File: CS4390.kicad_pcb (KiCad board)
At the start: 2 copper layers, 97.3 x 51.6 mm, 53 parts, among them J1 Power In, J2 Audio Out, J3 Data In, U1 CS4390, U2 OPA2604, U3 DRV134, U4 DRV134

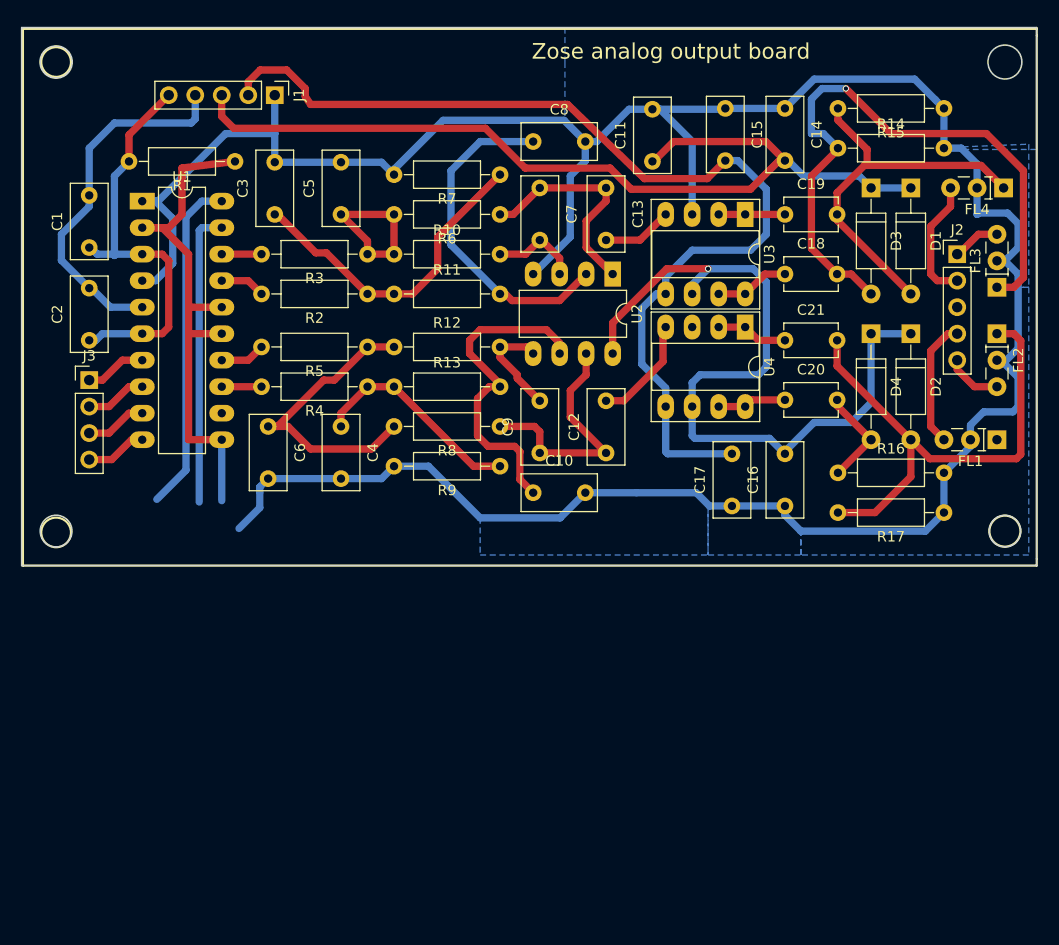
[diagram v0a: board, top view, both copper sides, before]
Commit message: pre-trace
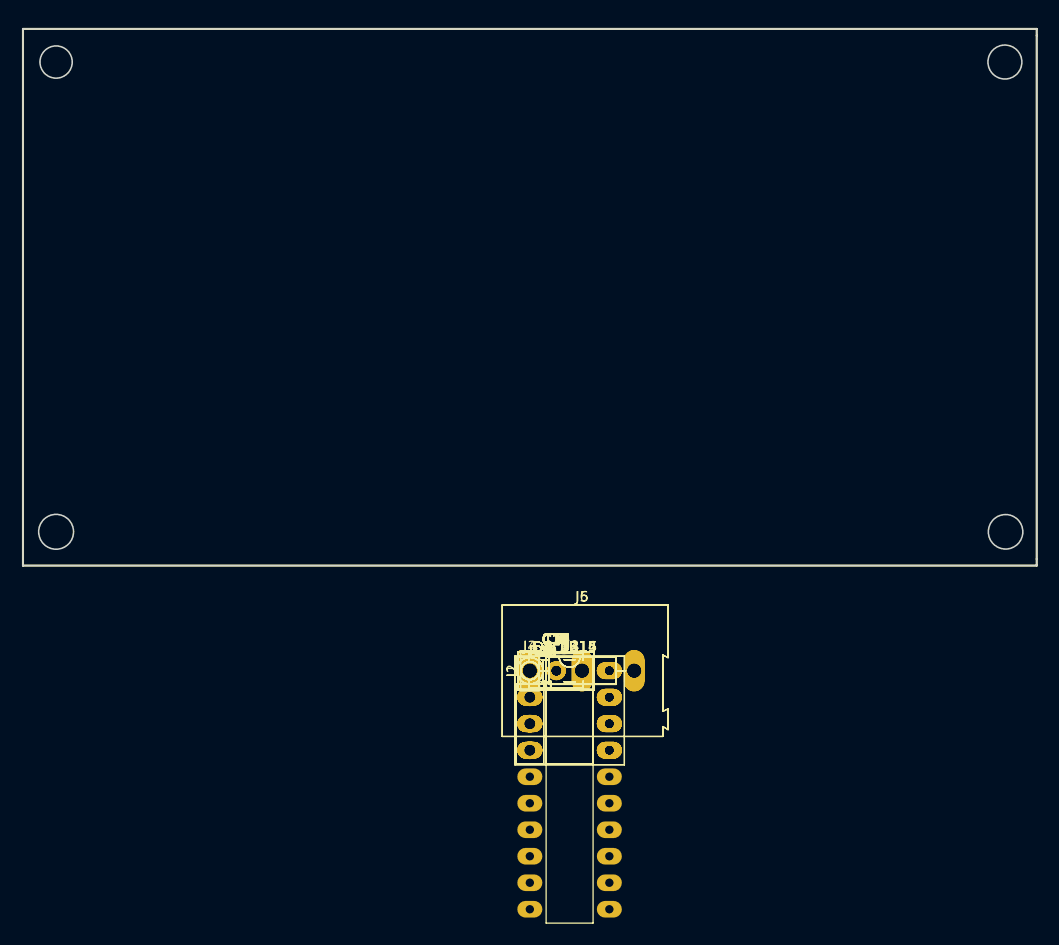
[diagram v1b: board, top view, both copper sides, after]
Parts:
- added J4: Power In, Pin_Headers:Pin_Header_Straight_1x04_Pitch2.54mm, F.Cu at (153.4, 133.3)
- added J5: Left, Connectors_Terminal_Blocks:TerminalBlock_Altech_AK300-3_P5.00mm, F.Cu at (153.4, 133.3)
- added J6: Right, Connectors_Terminal_Blocks:TerminalBlock_Altech_AK300-3_P5.00mm, F.Cu at (153.4, 133.3)
- C11: value 0.1uF -> 220pF
- C2: value 10uF -> 0.1uF
- C3: value 1nF -> 10uF
- C7: value 220pF -> 1nF
- D1, D2, D3, D4: footprint Diodes_THT:D_A-405_P10.16mm_Horizontal -> Diodes_THT:D_DO-35_SOD27_P2.54mm_Vertical_AnodeUp
- J1: value Power In -> GS3; footprint Pin_Headers:Pin_Header_Straight_1x05_Pitch2.54mm -> Connectors:GS3
- J2: value Audio Out -> GS3; footprint Pin_Headers:Pin_Header_Straight_1x05_Pitch2.54mm -> Connectors:GS3
- R1, R10, R11, R12, R13, R2, R3, R4, R5, R6, R7, R8, R9: footprint Resistors_THT:R_Axial_DIN0207_L6.3mm_D2.5mm_P10.16mm_Horizontal -> Resistors_THT:R_Axial_DIN0204_L3.6mm_D1.6mm_P2.54mm_Vertical
- U1: value CS4390 -> OPA2604; footprint Housings_DIP:DIP-20_W7.62mm_LongPads -> Housings_DIP:DIP-8_W7.62mm_LongPads
- U2: value OPA2604 -> CS4390; footprint Housings_DIP:DIP-8_W7.62mm_LongPads -> Housings_DIP:DIP-20_W7.62mm_LongPads
- moved R15 66.9 mm to (153.4, 133.3), turned to 0 degrees
- moved FL4 64.8 mm to (153.4, 133.3), turned to 0 degrees
- moved J1 60.3 mm to (153.4, 133.3), turned to 0 degrees
- moved C14 59.2 mm to (153.4, 133.3), turned to 0 degrees
- moved D1 58.9 mm to (153.4, 133.3), turned to 0 degrees
- moved C1 58.5 mm to (153.4, 133.3), turned to 0 degrees
- moved U1 58.4 mm to (153.4, 133.3)
- moved R14 58.1 mm to (153.4, 133.3)
- moved FL3 57.9 mm to (153.4, 133.3), turned to 0 degrees
- moved J2 57.2 mm to (153.4, 133.3)
- moved C15 57.1 mm to (153.4, 133.3), turned to 0 degrees
- moved D3 56.7 mm to (153.4, 133.3), turned to 0 degrees
- moved R1 56.4 mm to (153.4, 133.3), turned to 0 degrees
- moved FL2 55.2 mm to (153.4, 133.3), turned to 0 degrees
- moved C2 52.8 mm to (153.4, 133.3), turned to 0 degrees
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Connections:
- C1 pad 1: +5V -> +15V
- C1 pad 2: GND -> -12V
- C10 pad 2: GNDA -> Net-(C10-Pad2)
- C11 pad 1: +12V -> Net-(C11-Pad1)
- C13 pad 1: Net-(C13-Pad1) -> Net-(C10-Pad1)
- C14 pad 2: +12V -> +15V
- C16 pad 2: +12V -> +15V
- C2 pad 2: GND -> GNDA
- C3 pad 1: Net-(C3-Pad1) -> +5V
- C7 pad 1: Net-(C13-Pad1) -> Net-(C7-Pad1)
- C7 pad 2: Net-(C7-Pad2) -> GNDA
- C8 pad 1: Net-(C8-Pad1) -> Net-(C12-Pad1)
- C8 pad 2: GNDA -> Net-(C8-Pad2)
- C9 pad 1: Net-(C12-Pad1) -> Net-(C9-Pad1)
- C9 pad 2: Net-(C9-Pad2) -> GNDA
- D1 pad 1: +12V -> +15V
- D2 pad 1: +12V -> +15V
- D3 pad 1: +12V -> +15V
- D4 pad 1: +12V -> +15V
- FL1 pad 1: Net-(C20-Pad2) -> Net-(C18-Pad2)
- FL1 pad 3: R+ -> Net-(FL1-Pad3)
- FL2 pad 1: Net-(C21-Pad2) -> Net-(C19-Pad2)
- FL2 pad 3: R- -> Net-(FL2-Pad3)
- FL3 pad 1: Net-(C18-Pad2) -> Net-(C20-Pad2)
- FL3 pad 3: L+ -> Net-(FL3-Pad3)
- FL4 pad 1: Net-(C19-Pad2) -> Net-(C21-Pad2)
- FL4 pad 3: L- -> Net-(FL4-Pad3)
- J1 pad 1: GNDA -> Net-(J1-Pad1)
- J1 pad 2: -12V -> Net-(J1-Pad2)
- J1 pad 3: +12V -> GNDA
- J2 pad 1: L+ -> Net-(J1-Pad1)
- J2 pad 2: L- -> Net-(J2-Pad2)
- J2 pad 3: (no net) -> GNDA
- R1 pad 1: Net-(R1-Pad1) -> Net-(J1-Pad1)
- R10 pad 1: Net-(C5-Pad1) -> Net-(C6-Pad1)
- R10 pad 2: Net-(C7-Pad2) -> Net-(C8-Pad2)
- R11 pad 1: Net-(C3-Pad1) -> Net-(C4-Pad1)
- R11 pad 2: Net-(C8-Pad1) -> Net-(C9-Pad1)
- R12 pad 1: Net-(C6-Pad1) -> Net-(C7-Pad1)
- R12 pad 2: Net-(C9-Pad2) -> Net-(C10-Pad2)
- R13 pad 1: Net-(C4-Pad1) -> Net-(C5-Pad1)
- R13 pad 2: Net-(C10-Pad1) -> Net-(C11-Pad1)
- R2 pad 1: Net-(C3-Pad1) -> Net-(C6-Pad1)
- R3 pad 1: Net-(C5-Pad1) -> Net-(C4-Pad1)
- R4 pad 1: Net-(C4-Pad1) -> Net-(C7-Pad1)
- R5 pad 1: Net-(C6-Pad1) -> Net-(C5-Pad1)
- R6 pad 1: Net-(C13-Pad1) -> Net-(C12-Pad1)
- R6 pad 2: Net-(C5-Pad1) -> Net-(C6-Pad1)
- R7 pad 1: Net-(C3-Pad1) -> Net-(C4-Pad1)
- R8 pad 1: Net-(C12-Pad1) -> Net-(C10-Pad1)
- R8 pad 2: Net-(C6-Pad1) -> Net-(C7-Pad1)
- R9 pad 1: Net-(C4-Pad1) -> Net-(C5-Pad1)
- U1 pad 1: GNDA -> Net-(C10-Pad1)
- U1 pad 2: Net-(R1-Pad1) -> Net-(C10-Pad2)
- U1 pad 3: +5V -> Net-(C11-Pad1)
- U1 pad 4: GNDA -> -12V
- U1 pad 5: GND -> Net-(C9-Pad1)
- U1 pad 6: +5V -> Net-(C8-Pad2)
- U1 pad 7: LRCK -> Net-(C12-Pad1)
- U1 pad 8: MCLK -> +15V
- U2 pad 1: Net-(C13-Pad1) -> GNDA
- U2 pad 2: Net-(C8-Pad1) -> Net-(J1-Pad1)
- U2 pad 3: Net-(C7-Pad2) -> +5V
- U2 pad 5: Net-(C9-Pad2) -> GNDA
- U2 pad 6: Net-(C10-Pad1) -> +5V
- U2 pad 7: Net-(C12-Pad1) -> LRCK
- U2 pad 8: +12V -> MCLK
- U3 pad 4: Net-(C13-Pad2) -> Net-(C12-Pad2)
- U3 pad 6: +12V -> +15V
- U4 pad 3: (no net) -> GNDA
- U4 pad 4: Net-(C12-Pad2) -> Net-(C13-Pad2)
- U4 pad 6: +12V -> +15V
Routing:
- net GNDA: track 262.1 -> 0.00 mm
- net +12V: track 162.2 -> 0.00 mm, vias 1 -> 0
- net -12V: track 99.3 -> 0.00 mm
- net Net-(C18-Pad2): track 61.8 -> 0.00 mm, vias 1 -> 0
- net (no net): track 60.6 -> 0.00 mm
- net Net-(R1-Pad1): track 52.5 -> 0.00 mm
- net Net-(C21-Pad2): track 49.3 -> 0.00 mm
- net +5V: track 40.3 -> 0.00 mm
- net Net-(C19-Pad2): track 37.2 -> 0.00 mm
- net GND: track 35.1 -> 0.00 mm
- net Net-(C8-Pad1): track 32.4 -> 0.00 mm
- net Net-(C10-Pad1): track 31.6 -> 0.00 mm
- net Net-(C3-Pad1): track 31.3 -> 0.00 mm
- net Net-(C6-Pad1): track 29.1 -> 0.00 mm
- net Net-(C12-Pad1): track 24.0 -> 0.00 mm
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- removed copper zone on B.Cu, net GNDA
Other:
- board size 97.3 x 51.6 mm -> 97.2 x 51.4 mm
- board text removed: "Zose analog output board"

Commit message: base placement
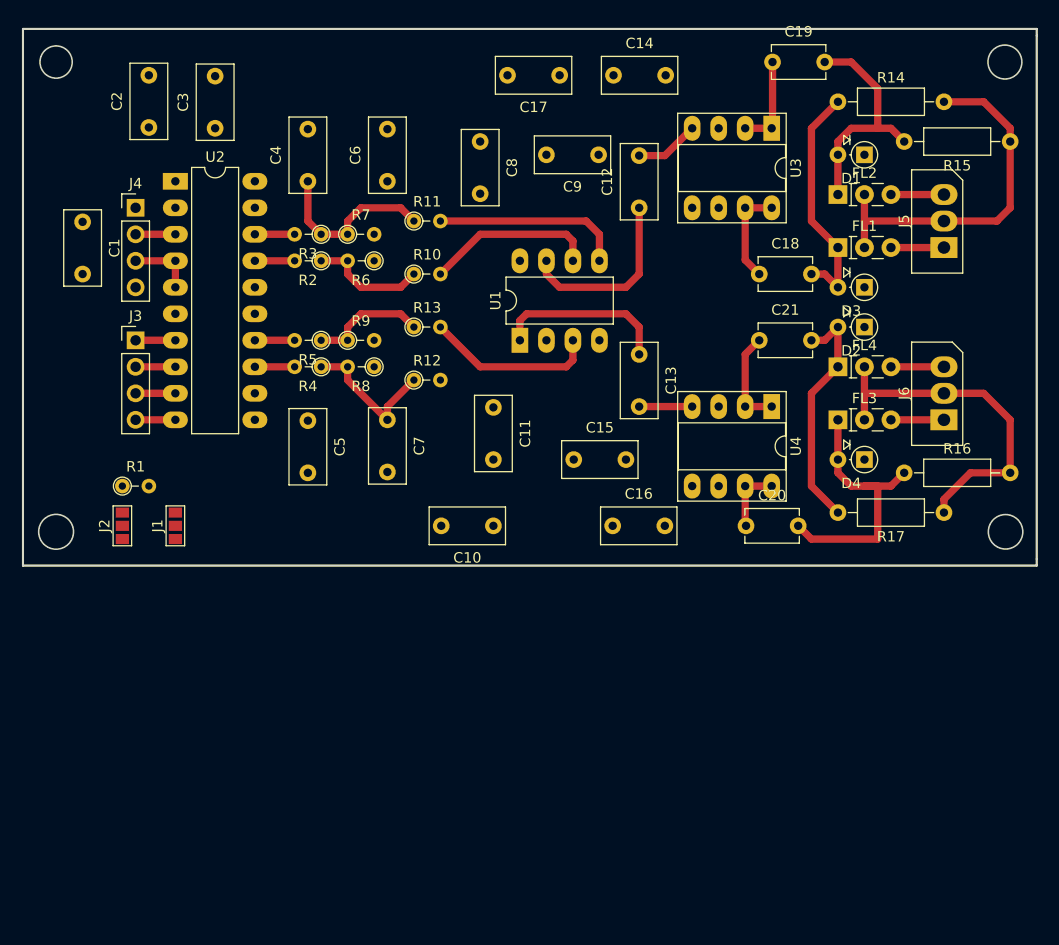
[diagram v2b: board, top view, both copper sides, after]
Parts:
- J5, J6: footprint Connectors_Terminal_Blocks:TerminalBlock_Altech_AK300-3_P5.00mm -> Connectors_Molex:Molex_SPOX-5267_22-03-5035_03x2.54mm_Straight
- moved R15 68.5 mm to (199.4, 82.5), turned to 180 degrees
- moved C2 63.6 mm to (116.8, 81.2), turned to 90 degrees
- moved C19 62.8 mm to (176.6, 74.9)
- moved R14 62.0 mm to (182.9, 78.7)
- moved C1 60.7 mm to (110.5, 90.2), turned to 270 degrees
- moved C3 60.1 mm to (123.2, 81.3), turned to 90 degrees
- moved D1 58.9 mm to (185.4, 83.8), turned to 180 degrees
- moved J4 58.3 mm to (115.6, 88.9)
- moved U2 57.9 mm to (119.4, 86.4)
- moved C14 57.6 mm to (161.4, 76.2)
- moved C17 57.1 mm to (156.2, 76.2), turned to 180 degrees
- moved U3 56.9 mm to (176.5, 81.3), turned to 270 degrees
- moved J5 56.7 mm to (193.0, 92.7), turned to 90 degrees
- moved FL2 54.4 mm to (182.9, 87.6)
- moved C4 51.5 mm to (132.1, 86.4), turned to 90 degrees
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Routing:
- net GNDA: track 0.00 -> 74.8 mm
- net Net-(C20-Pad2): track 0.00 -> 27.0 mm
- net Net-(C18-Pad2): track 0.00 -> 23.0 mm
- net Net-(C21-Pad2): track 0.00 -> 23.0 mm
- net Net-(C19-Pad2): track 0.00 -> 22.4 mm
- net Net-(C9-Pad1): track 0.00 -> 18.3 mm
- net Net-(C12-Pad1): track 0.00 -> 17.6 mm
- net Net-(C4-Pad1): track 0.00 -> 16.8 mm
- net Net-(C10-Pad1): track 0.00 -> 16.7 mm
- net Net-(C8-Pad2): track 0.00 -> 16.4 mm
- net Net-(C11-Pad1): track 0.00 -> 16.4 mm
- net Net-(C7-Pad1): track 0.00 -> 14.1 mm
- net Net-(C6-Pad1): track 0.00 -> 11.2 mm
- net Net-(C5-Pad1): track 0.00 -> 11.2 mm
- net Net-(C21-Pad1): track 0.00 -> 9.45 mm
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
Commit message: gerber
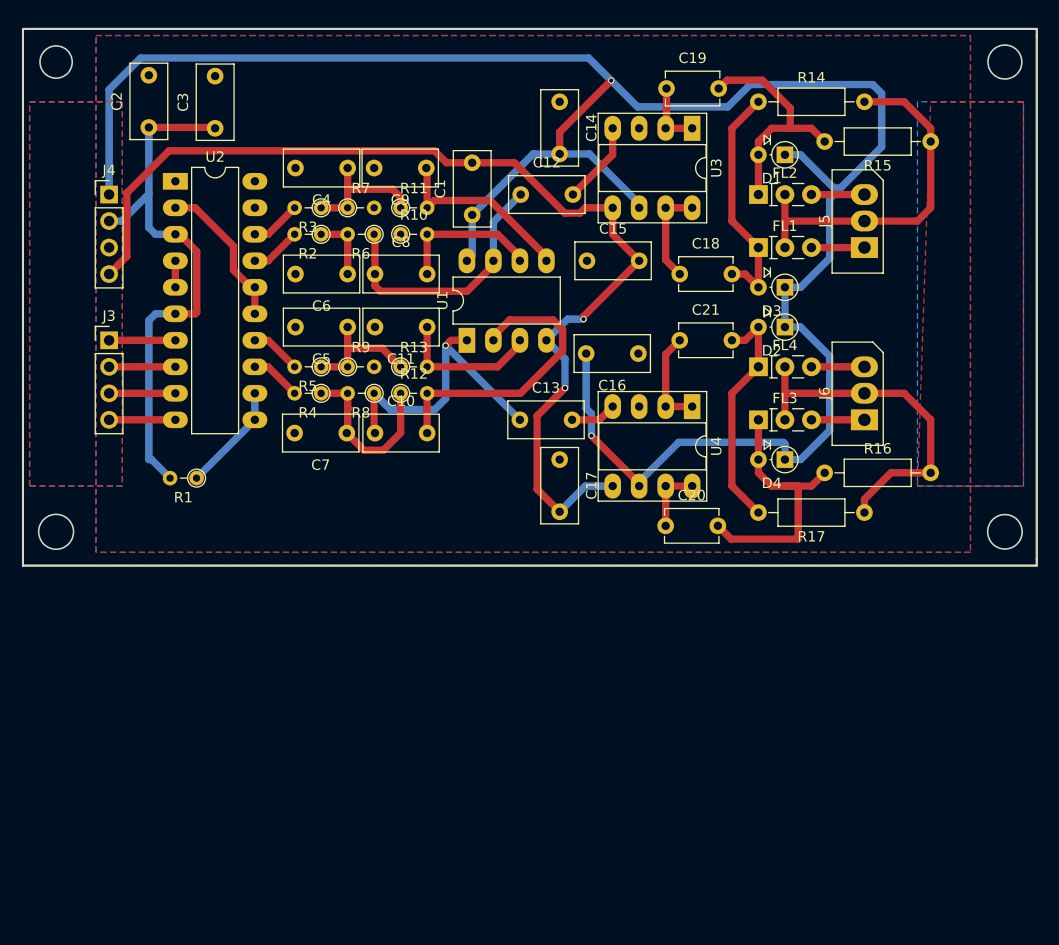
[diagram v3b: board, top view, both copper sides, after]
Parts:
- removed J1, J2: GS3, Connectors:GS3
- moved C1 37.3 mm to (147.8, 89.6), turned to 90 degrees
- moved C17 36.8 mm to (156.2, 113.0), turned to 270 degrees
- moved C15 19.1 mm to (158.8, 94.0)
- moved C16 16.7 mm to (163.8, 102.9), turned to 180 degrees
- moved C9 16.6 mm to (143.4, 85.1)
- moved C8 16.2 mm to (138.5, 95.2), turned to 0 degrees
- moved C10 14.4 mm to (138.5, 110.5), turned to 0 degrees
- moved C13 13.0 mm to (152.4, 109.2), turned to 0 degrees
- moved C12 11.4 mm to (152.5, 87.6), turned to 0 degrees
- moved C19 10.5 mm to (166.4, 77.5)
- moved C11 9.98 mm to (143.5, 100.3), turned to 180 degrees
- moved C5 9.75 mm to (135.9, 100.3), turned to 180 degrees
- moved C6 9.67 mm to (135.9, 95.2), turned to 180 degrees
- moved C20 7.70 mm to (166.4, 119.4)
- moved C18 7.62 mm to (167.7, 95.2)
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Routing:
- net +15V: track 0.00 -> 207.1 mm, vias 0 -> 2
- net -12V: track 0.00 -> 103.0 mm, vias 0 -> 2
- net +5V: track 3.81 -> 53.2 mm
- net Net-(C10-Pad2): track 0.00 -> 28.8 mm
- net Net-(J1-Pad1): track 0.00 -> 25.1 mm
- net Net-(C10-Pad1): track 16.7 -> 29.2 mm, vias 0 -> 1
- net Net-(C12-Pad1): track 17.6 -> 25.4 mm
- net Net-(C6-Pad1): track 11.2 -> 6.35 mm
- net Net-(C4-Pad1): track 16.8 -> 12.7 mm
- net Net-(C7-Pad1): track 14.1 -> 16.8 mm
- net GNDA: track 74.8 -> 72.1 mm
- net SDATA: track 3.81 -> 6.35 mm
- net MCLK: track 3.81 -> 6.35 mm
- net LRCK: track 3.81 -> 6.35 mm
- net BCLK: track 3.81 -> 6.35 mm
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- added copper zone on B.Cu, net GNDA
- added copper zone on F.Cu, net GNDA
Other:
- net class Default: clearance 0.2 -> 0.5
- rule trace_clearance: 0.2 -> 0.5
